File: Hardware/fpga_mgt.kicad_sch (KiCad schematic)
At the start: 1 part, among them U1 XC7A50T-CPG236

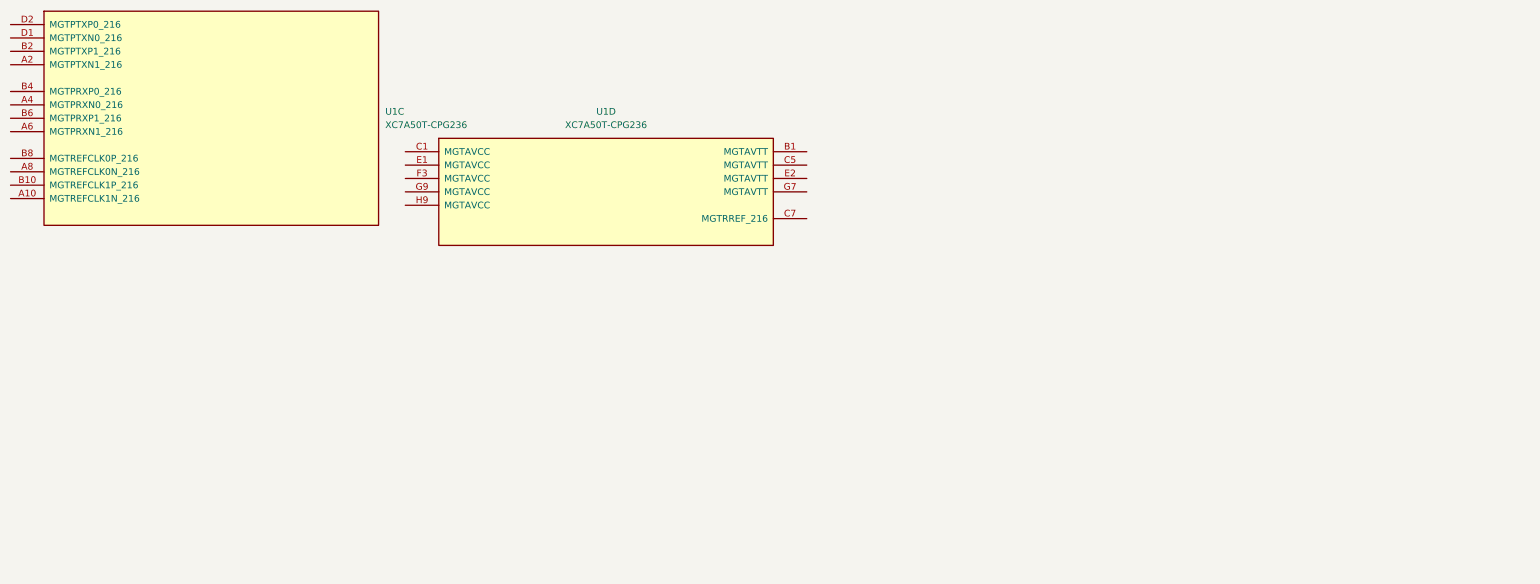
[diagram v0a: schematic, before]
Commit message: CSG325?
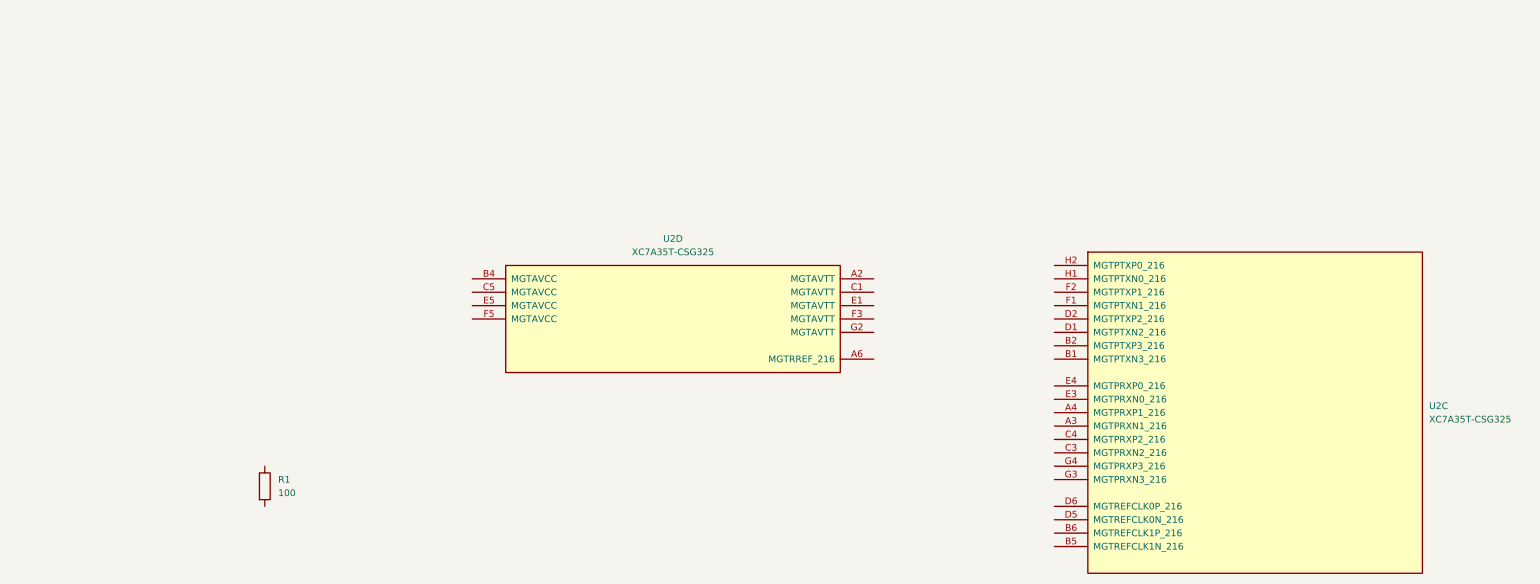
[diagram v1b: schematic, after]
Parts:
- removed U1: XC7A50T-CPG236, Package_BGA:Xilinx_CPG236, symbol FPGA_Xilinx_Artix7:XC7A50T-CPG236
- added R1: 100, Resistor_SMD:R_0402_1005Metric, symbol Device:R
- added U2: XC7A35T-CSG325, Package_BGA:Xilinx_CSG325, symbol FPGA_Xilinx_Artix7:XC7A35T-CSG325
